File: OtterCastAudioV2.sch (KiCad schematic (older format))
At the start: 24 parts, among them J1 UART, J2 SD, U1 AllWinner-S3(FBGA-234), U2 AT24CS16-MAHM

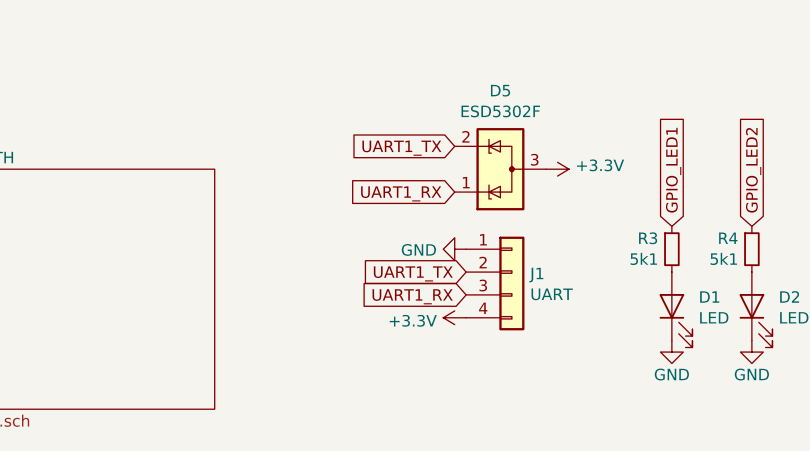
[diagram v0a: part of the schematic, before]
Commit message: update
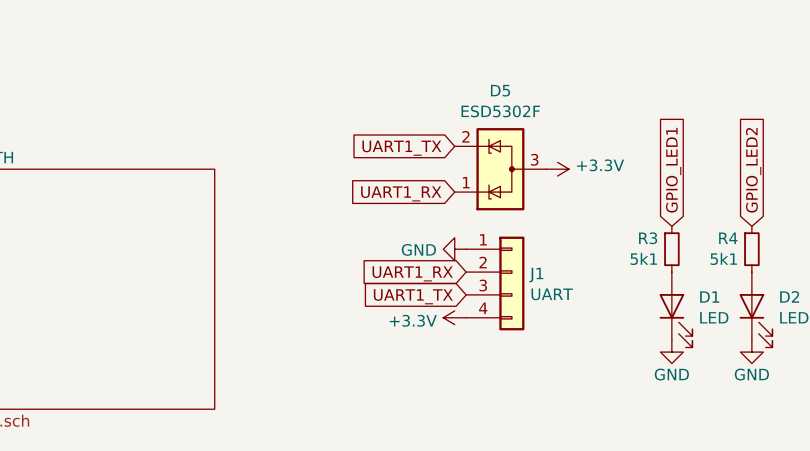
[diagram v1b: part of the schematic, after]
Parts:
- J1: footprint Connector_PinHeader_2.00mm:PinHeader_1x04_P2.00mm_Vertical -> otter:PinHeader_1x04_P2.00mm_Vertical_nosilk_center
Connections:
- net UART1_RX: now also J1.2 (Pin_2); no longer J1.3 (Pin_3)
- net UART1_TX: now also J1.3 (Pin_3); no longer J1.2 (Pin_2)
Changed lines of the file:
@@
 F 0 "J1" H 7480 10392 50  0000 L CNN
 F 1 "UART" H 7480 10301 50  0000 L CNN
-F 2 "Connector_PinHeader_2.00mm:PinHeader_1x04_P2.00mm_Vertical" H 7400 10400 50  0001 C CNN
+F 2 "otter:PinHeader_1x04_P2.00mm_Vertical_nosilk_center" H 7400 10400 50  0001 C CNN
 F 3 "~" H 7400 10400 50  0001 C CNN
 	1    7400 10400
@@
 	0    1    1    0
 $EndComp
+Text GLabel 7200 10500 0    50   Input ~ 0
+UART1_TX
 Text GLabel 7200 10400 0    50   Input ~ 0
-UART1_TX
-Text GLabel 7200 10500 0    50   Input ~ 0
 UART1_RX
 $Comp
